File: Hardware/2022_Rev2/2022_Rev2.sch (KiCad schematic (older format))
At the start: 16 parts

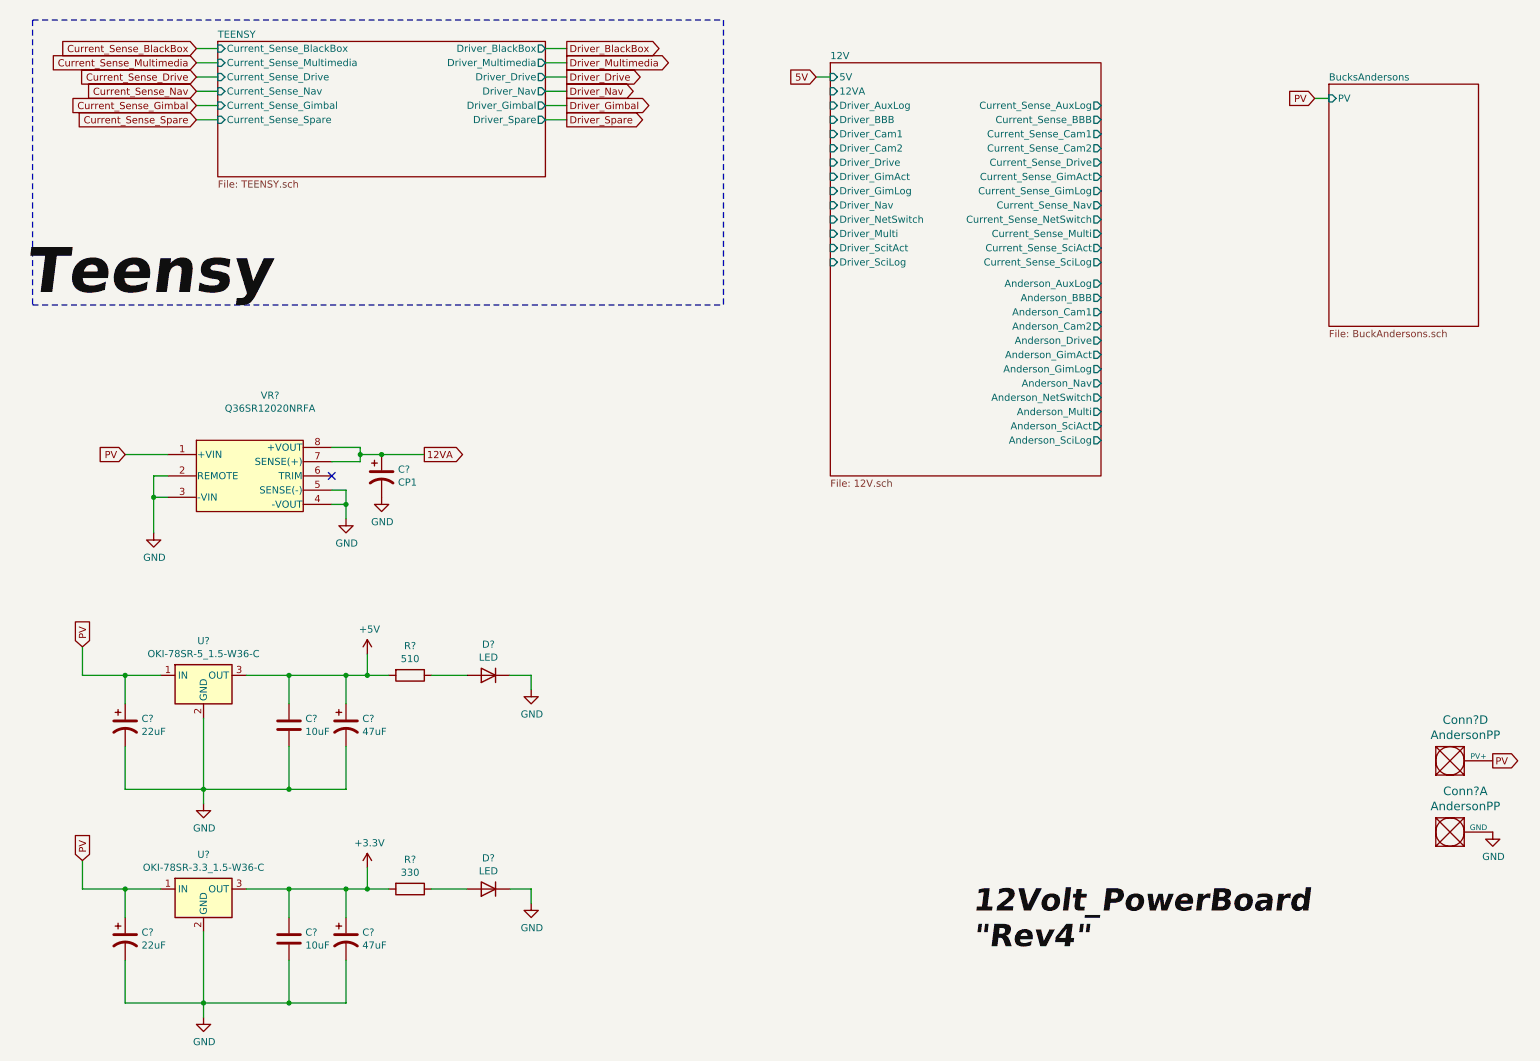
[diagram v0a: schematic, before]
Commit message: andersons done
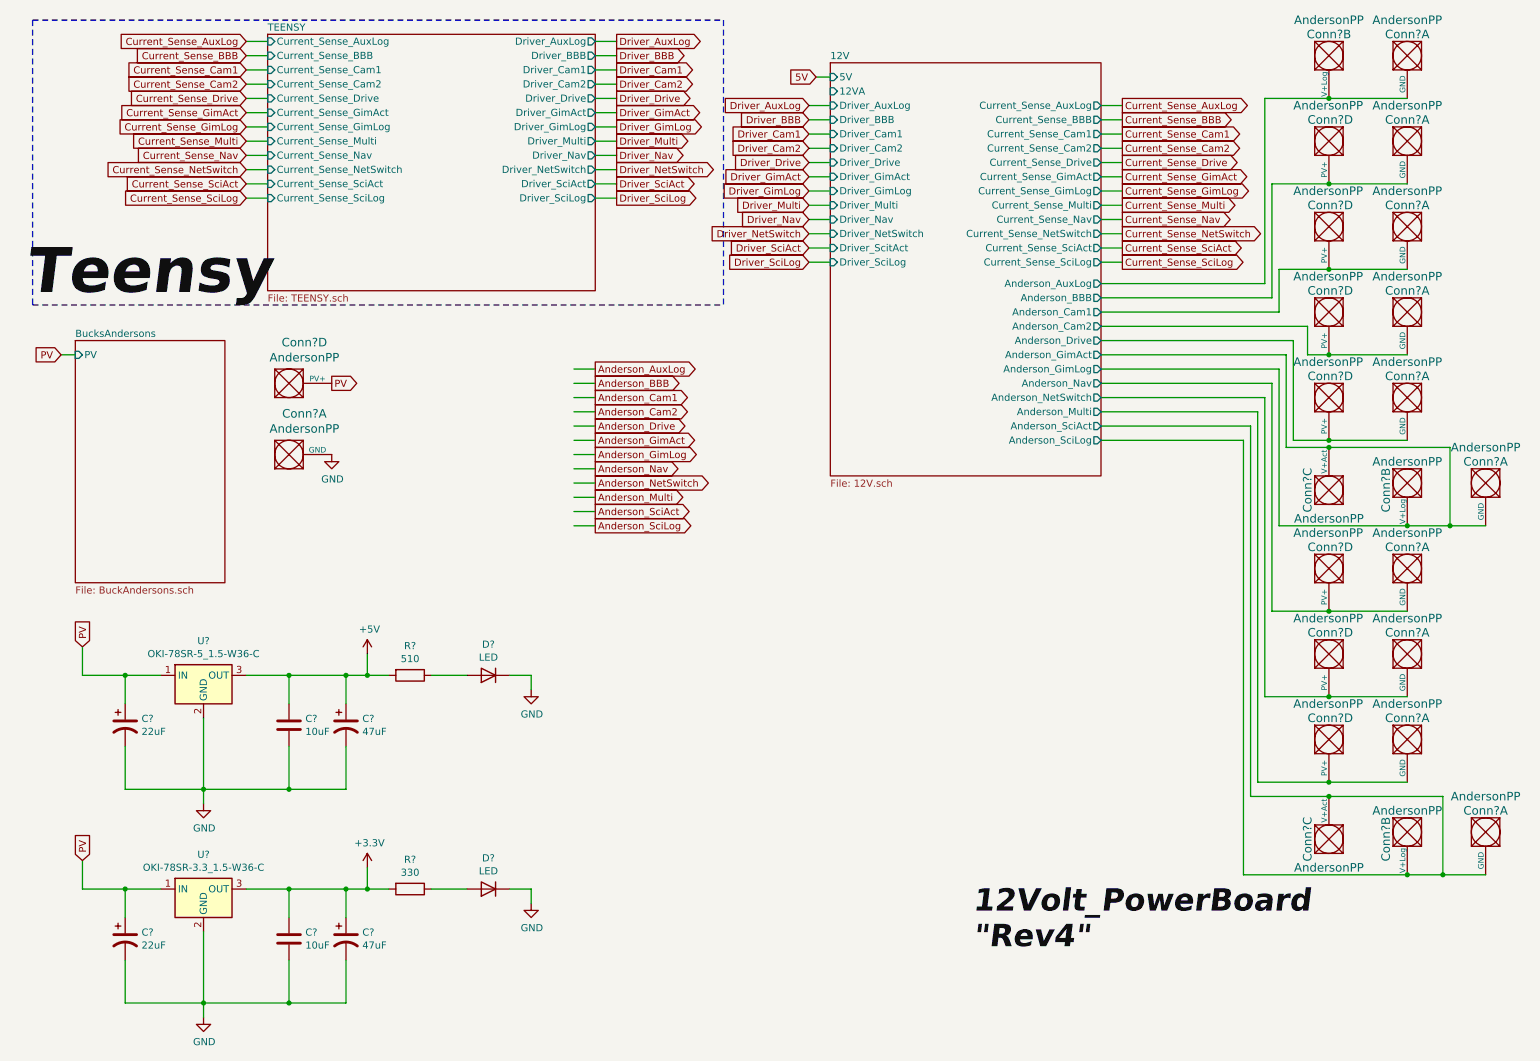
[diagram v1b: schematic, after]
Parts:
- removed C?: CP1, symbol Device:CP1
- removed VR?: Q36SR12020NRFA, symbol MRDT_Devices:Q36SR12020NRFA
- added Conn? (x22): AndersonPP, symbol MRDT_Connectors:AndersonPP
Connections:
- net labels added: Anderson_AuxLog, Anderson_BBB, Anderson_Cam1, Anderson_Cam2, Anderson_Drive, Anderson_GimAct, Anderson_GimLog, Anderson_Multi, Anderson_Nav, Anderson_NetSwitch, Anderson_SciAct, Anderson_SciLog, Current_Sense_AuxLog, Current_Sense_BBB, Current_Sense_Cam1, Current_Sense_Cam2, Current_Sense_GimAct, Current_Sense_GimLog, Current_Sense_Multi, Current_Sense_NetSwitch, Current_Sense_SciAct, Current_Sense_SciLog, Driver_AuxLog, Driver_BBB, Driver_Cam1, Driver_Cam2, Driver_GimAct, Driver_GimLog, Driver_Multi, Driver_NetSwitch, Driver_SciAct, Driver_SciLog
- net labels removed: 12VA, Current_Sense_BlackBox, Current_Sense_Gimbal, Current_Sense_Multimedia, Current_Sense_Spare, Driver_BlackBox, Driver_Gimbal, Driver_Multimedia, Driver_Spare
- wire segments 73 -> 158
- no-connect marks 1 -> 0
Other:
- moved on the sheet: Conn?A, Conn?D
